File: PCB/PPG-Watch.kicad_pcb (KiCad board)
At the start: 6 copper layers, 21 x 36 mm, 79 parts, among them J1 USB_C_Receptacle_USB2.0_16P, Q1 RE1C002UN, Q2 SI2302CDS, Q3 RE1C002ZP, Q4 RE1C002UN, Q5 RE1C002UN, Q6 RE1C002UN, Q7 RE1C002UN, U1 LSM6DSM, U10 MCP3561R, U11 MCP23S18x-x-MJ, U2 nRF52833_QDxx, U3 MCP73832-2-OT, U4 OPA2381, U5 SR4W035, U6 TPS78227DDC, U7 TXU0102, U8 NJL5821R, Y1 SiT1552

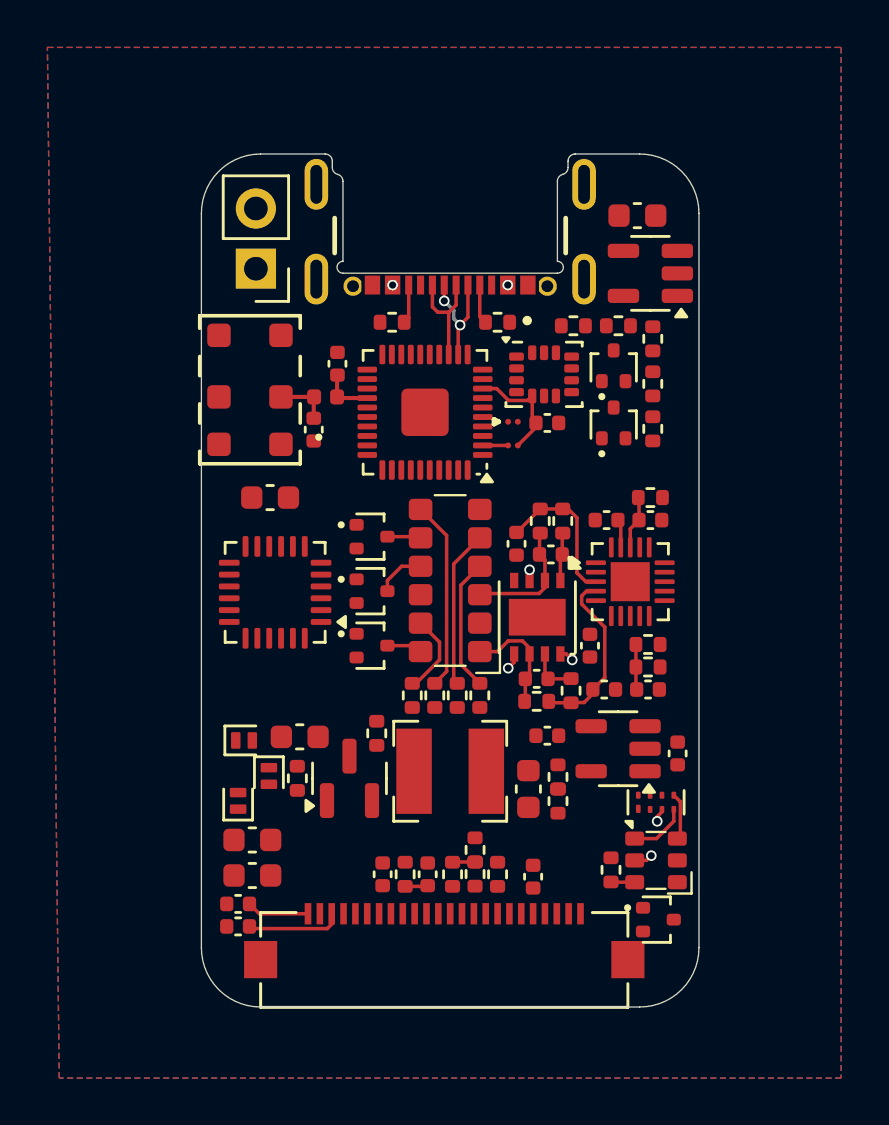
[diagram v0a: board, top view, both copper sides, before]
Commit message: layout complete!!!
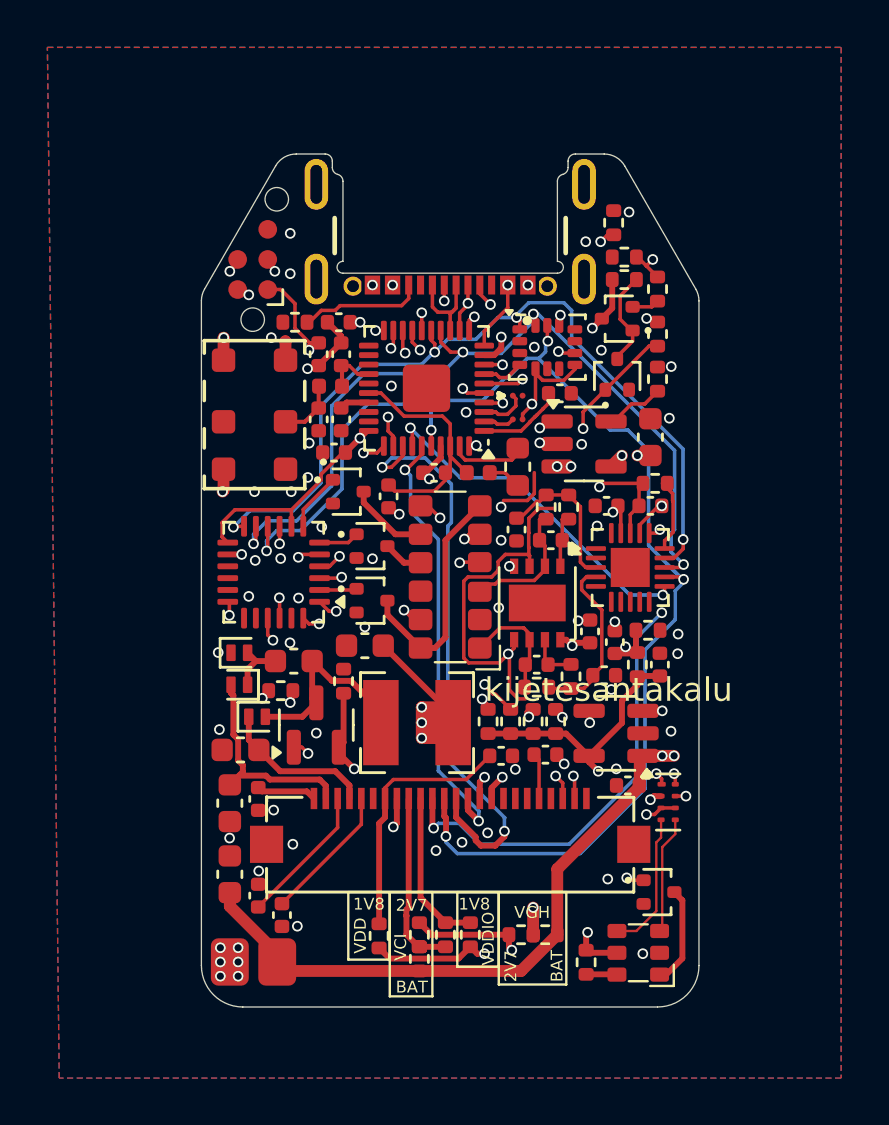
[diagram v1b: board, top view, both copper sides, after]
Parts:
- added C23: 1u, Capacitor_SMD:C_0402_1005Metric, F.Cu at (45.3, 37.1)
- added C28: 100n, Capacitor_SMD:C_0402_1005Metric, F.Cu at (44.5, 38.5)
- added C29: 100n, Capacitor_SMD:C_0402_1005Metric, F.Cu at (54.6, 40.1)
- added C30: 100p, Capacitor_SMD:C_0402_1005Metric, F.Cu at (45.4, 41.2)
- added C31: 47n, Capacitor_SMD:C_0402_1005Metric, F.Cu at (47.4, 44.5)
- added C32: 1u, Capacitor_SMD:C_0402_1005Metric, F.Cu at (49.3, 43.5)
- added J2: Conn_ARM_SWD_TagConnect_TC2030-NL, Connector:Tag-Connect_TC2030-IDC-NL_2x03_P1.27mm_Vertical, F.Cu at (41.7, 34.5)
- added L3: 10u, Inductor_SMD:L_0603_1608Metric, F.Cu at (52.9, 43.2)
- added L4: 15n, Inductor_SMD:L_0402_1005Metric, F.Cu at (51.2, 43.5)
- BT1: footprint Connector_PinHeader_2.54mm:PinHeader_1x02_P2.54mm_Vertical -> Library:Battery
- C14: value C -> 1p2
- C8: value C -> 1p5
- L2: value L -> 4n2
- moved BT1 29.3 mm to (41.7, 64.1)
- moved C4 16.0 mm to (40.7, 60.4), turned to 90 degrees
- moved DIS1 10.8 mm to (50.0, 58.7)
- moved C5 9.37 mm to (58.5, 42.0), turned to 90 degrees
- moved C1 9.18 mm to (46.4, 50.8), turned to 180 degrees
- moved C26 9.09 mm to (45.1, 42.6), turned to 180 degrees
- moved U3 7.73 mm to (55.6, 42.2), turned to 0 degrees
- moved R29 6.84 mm to (53.0, 63.0), turned to 0 degrees
- moved R7 6.45 mm to (56.9, 32.9), turned to -90 degrees
- moved C13 5.88 mm to (52.1, 55.4), turned to 180 degrees
- moved R28 5.67 mm to (54.0, 63.0), turned to 180 degrees
- moved C7 5.62 mm to (58.9, 51.5), turned to 90 degrees
- moved C16 5.18 mm to (54.0, 55.4), turned to 0 degrees
- moved C12 4.58 mm to (42.9, 62.1), turned to 90 degrees
- moved R1 4.56 mm to (57.4, 35.3), turned to 0 degrees
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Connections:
- DIS1 pad GND1: unconnected-(DIS1-PadGND1) -> GND
- DIS1 pad GND2: unconnected-(DIS1-PadGND2) -> GND
- U10 pad 16: unconnected-(U10-MCLK-Pad16) -> /MCLK
- U11 pad 1: unconnected-(U11-GPB1-Pad1) -> /enc_A
- U11 pad 13: unconnected-(U11-~{RESET}-Pad13) -> +1V8
- U11 pad 14: unconnected-(U11-INTA-Pad14) -> /Int
- U11 pad 18: unconnected-(U11-GPA3-Pad18) -> /enc_LED_en
- U11 pad 2: unconnected-(U11-GPB2-Pad2) -> /GLED_en
- U11 pad 21: unconnected-(U11-GPA6-Pad21) -> /RES
- U11 pad 22: unconnected-(U11-GPA7-Pad22) -> /BUSY
- U11 pad 24: unconnected-(U11-GPB0-Pad24) -> /enc_B
- U11 pad 3: unconnected-(U11-GPB3-Pad3) -> /2V7_en
- U11 pad 4: unconnected-(U11-GPB4-Pad4) -> /bat_mon_en
- U11 pad 5: unconnected-(U11-GPB5-Pad5) -> /charge_stat
- U11 pad 6: unconnected-(U11-GPB6-Pad6) -> /IRLED_en
- U11 pad 7: unconnected-(U11-GPB7-Pad7) -> /RLED_en
- U2 pad 1: unconnected-(U2-DEC1-Pad1) -> Net-(U2-DEC1)
- U2 pad 11: unconnected-(U2-DECUSB-Pad11) -> Net-(U2-DECUSB)
- U2 pad 14: unconnected-(U2-P0.15-Pad14) -> /CTX
- U2 pad 15: unconnected-(U2-P0.17-Pad15) -> /PTX
- U2 pad 16: unconnected-(U2-P0.18/~{RESET}-Pad16) -> Net-(J2-~{RESET})
- U2 pad 17: unconnected-(U2-P0.20-Pad17) -> /CS2
- U2 pad 19: unconnected-(U2-SWDIO-Pad19) -> Net-(J2-SWDIO)
- U2 pad 20: unconnected-(U2-SWDCLK-Pad20) -> Net-(J2-SWCLK)
- U2 pad 26: unconnected-(U2-DEC6-Pad26) -> Net-(U2-DEC4)
- U2 pad 27: unconnected-(U2-DEC3-Pad27) -> Net-(U2-DEC3)
- U2 pad 31: unconnected-(U2-AIN1/P0.03-Pad31) -> /Int
- U2 pad 32: unconnected-(U2-AIN0/P0.02-Pad32) -> /CS4
- U2 pad 33: unconnected-(U2-AIN4/P0.28-Pad33) -> /CS1
- U2 pad 34: unconnected-(U2-AIN5/P0.29-Pad34) -> /CS3
- U2 pad 35: unconnected-(U2-AIN6/P0.30-Pad35) -> /D/C
- U2 pad 36: unconnected-(U2-AIN7/P0.31-Pad36) -> /CLK
- U2 pad 38: unconnected-(U2-DEC4-Pad38) -> Net-(U2-DEC4)
- U2 pad 39: unconnected-(U2-DCC-Pad39) -> Net-(U2-DCC)
- U2 pad 4: unconnected-(U2-AIN2/P0.04-Pad4) -> /MCLK
- U2 pad 5: unconnected-(U2-AIN3/P0.05-Pad5) -> /bat_mon
- U2 pad 6: unconnected-(U2-P1.09-Pad6) -> /IMU_int2
- U2 pad 7: unconnected-(U2-P0.11-Pad7) -> /IMU_int1
- U4 pad 9: (no net) -> GND
- U7 pad 6: /enc_en -> +2V7
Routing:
- net +1V8: track 7.11 -> 82.9 mm, vias 0 -> 9
- net /CLK: track 0.00 -> 57.3 mm, vias 0 -> 5
- net /CTX: track 0.00 -> 56.9 mm, vias 0 -> 6
- net +BATT: track 0.00 -> 56.6 mm, vias 0 -> 6
- net +2V7: track 3.17 -> 46.4 mm, vias 3 -> 6
- net /PTX: track 0.00 -> 35.3 mm, vias 0 -> 4
- net /enc_LED_en: track 0.00 -> 24.6 mm, vias 0 -> 2
- net Net-(C1-Pad1): track 0.00 -> 24.5 mm, vias 0 -> 4
- net /CS1: track 0.00 -> 24.5 mm, vias 0 -> 2
- net VBUS: track 0.00 -> 20.4 mm, vias 2 -> 4
- net /trans_bias: track 3.07 -> 22.8 mm
- net /enc_B: track 0.00 -> 19.4 mm, vias 0 -> 2
- net /bat_mon_en: track 0.00 -> 19.0 mm, vias 0 -> 2
- net /D/C: track 0.00 -> 18.6 mm, vias 0 -> 2
- net /2V7_en: track 0.00 -> 18.5 mm, vias 0 -> 2
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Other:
- outline, holes or cut-outs redrawn
- board text added: "1V8"
- board text added: "2V7"
- board text added: "BAT"
- board text added: "Gavin Ford (11-25)"
- board text added: "My therapist: <has a pulse> Me (to myself): This is great. I'm going to get a good grade in photoplethysmography, something that is both normal to want and possible to achieve,"
- board text added: "VCI"
- board text added: "VDD"
- board text added: "VDDIO"
- board text added: "VGH"
- board text added: "kijetesantakalu"
- board text added: "this is a PPG smartwatch btw"
- board text removed: "TODO: Position flat flex encoder pos"
